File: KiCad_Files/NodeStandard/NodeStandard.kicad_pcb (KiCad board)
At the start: 2 copper layers, 105 parts, among them J1 AC Current In, J10 Opto Coupler 1 in, J11 Opto Coupler 2 in, J12 Opto Coupler 3 in, J13 Relay 1 Output, J14 Relay 2 Output, J15 Schakelaar 3 in, J16 Schakelaar 2 in, J17 Schakelaar 1 in, J18 Force output FET 1 on, J19 Force output FET 2 on, J2 AudioJack3_SwitchTR, J20 FET 1 Output, J21 FET 1 Output, J22 Force output Relay 3 on, J23 Relay 3 Output 1, J24 Relay 3 Output 2, J25 230VAC in, J26 5V-in, J27 ExtDC-in, J3 AC Current loop, J4 EXT1, J5 OledDisplay, J6 RFIDReader, J7 EXT2, J8 Force output Relay 1 on, J9 Force output Relay 2 on, K1 SANYOU_SRD_Form_C, K2 SANYOU_SRD_Form_C, K3 RT42xAxx, Q1 BC547, Q2 BC547, Q3 IRLZ34N, Q4 IRLZ34N, Q5 BC547, U1 MCP23017_SP

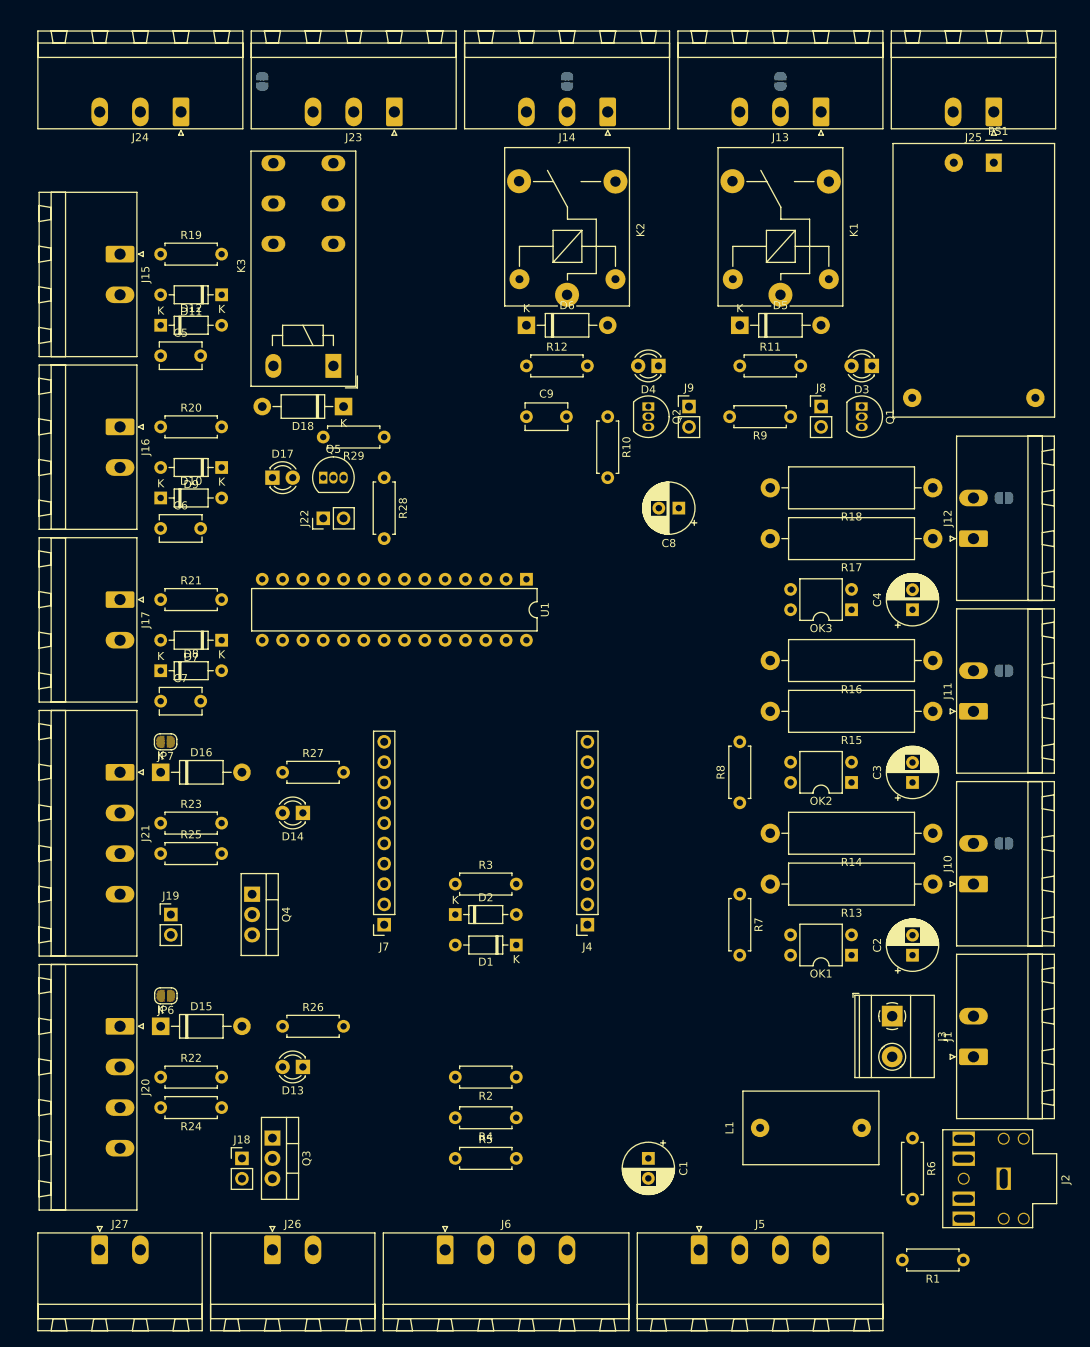
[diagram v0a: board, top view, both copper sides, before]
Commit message: V0.5 Work in progress, first version  PCB design, no silk screen yet
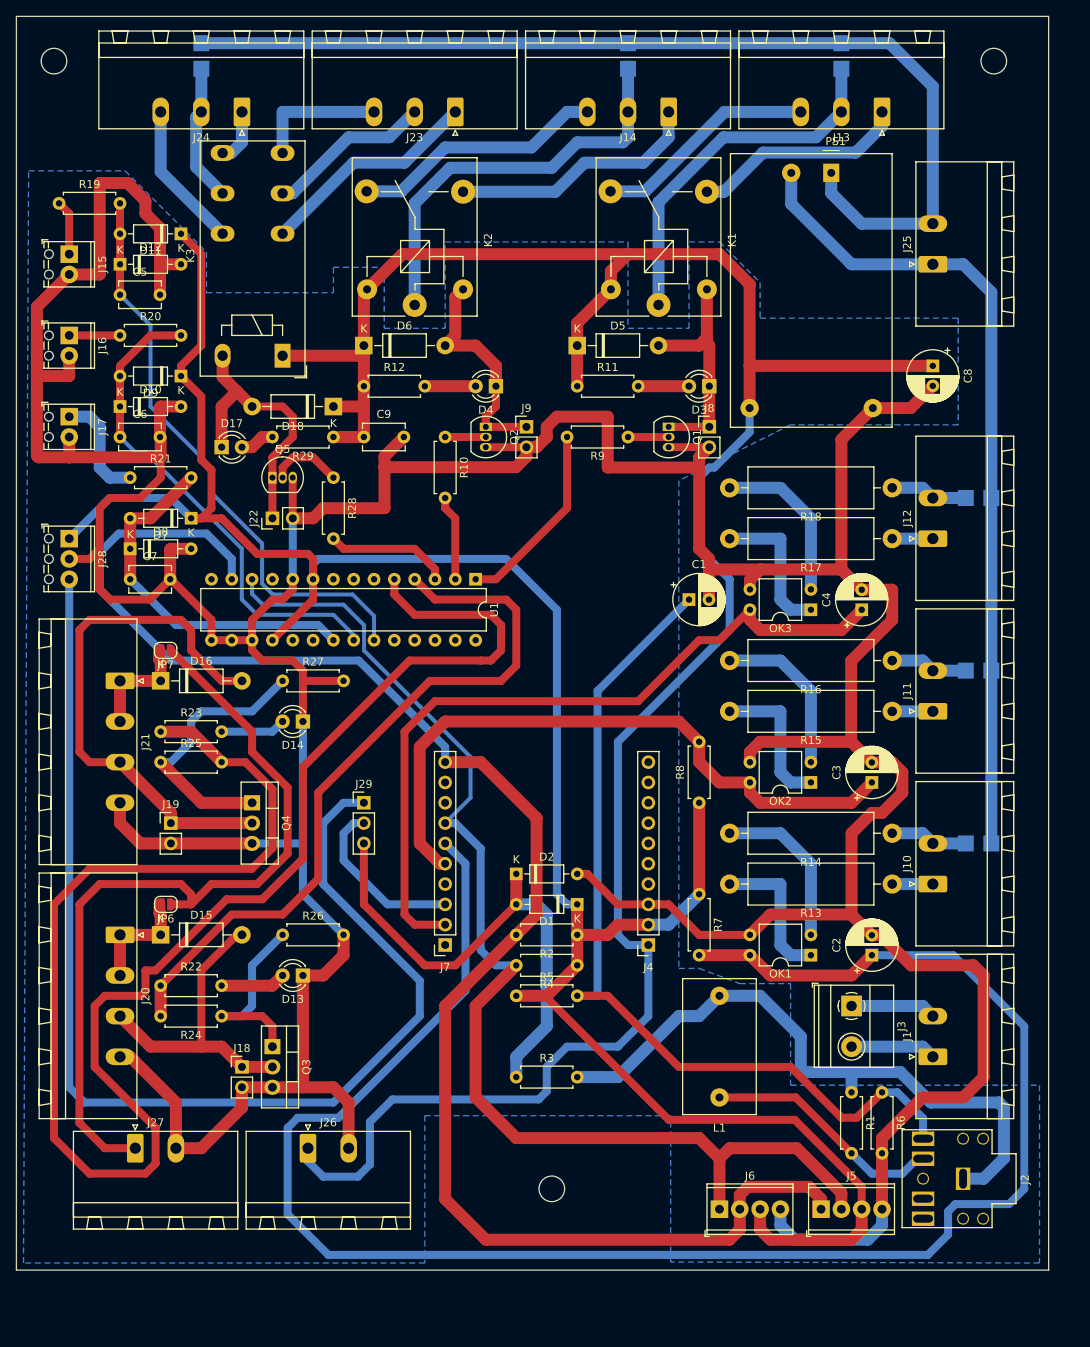
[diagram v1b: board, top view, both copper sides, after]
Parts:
- added J28: Hal current sensor, TerminalBlock_Phoenix:TerminalBlock_Phoenix_MPT-0,5-3-2.54_1x03_P2.54mm_Horizontal, F.Cu at (36.8, 86.4)
- added J29: Current sensor select, Connector_PinHeader_2.54mm:PinHeader_1x03_P2.54mm_Vertical, F.Cu at (73.7, 119.4)
- added REF**: MountingHole_3.2mm_M3, MountingHole:MountingHole_3.2mm_M3, F.Cu at (97.2, 167.6)
- added REF**: MountingHole_3.2mm_M3, MountingHole:MountingHole_3.2mm_M3, F.Cu at (152.4, 26.7)
- added REF**: MountingHole_3.2mm_M3, MountingHole:MountingHole_3.2mm_M3, F.Cu at (34.9, 26.7)
- J15, J16, J17: footprint Connector_Phoenix_MSTB:PhoenixContact_MSTB_2,5_2-GF-5,08_1x02_P5.08mm_Horizontal_ThreadedFlange -> TerminalBlock_Phoenix:TerminalBlock_Phoenix_MPT-0,5-2-2.54_1x02_P2.54mm_Horizontal
- J5, J6: footprint Connector_Phoenix_MSTB:PhoenixContact_MSTB_2,5_4-GF-5,08_1x04_P5.08mm_Horizontal_ThreadedFlange -> TerminalBlock_Phoenix:TerminalBlock_Phoenix_MPT-0,5-4-2.54_1x04_P2.54mm_Horizontal
- JP1, JP2, JP3, JP4, JP5, JP8: footprint Jumper:SolderJumper-2_P1.3mm_Open_RoundedPad1.0x1.5mm -> Footprints:SolderJumper-2_P3mm_Open_RoundedPad
- moved C1 70.0 mm to (114.3, 94.0), turned to 0 degrees
- moved C8 36.4 mm to (144.8, 64.8), turned to 270 degrees
- moved J6 34.7 mm to (118.1, 170.2)
- moved R3 25.3 mm to (92.7, 153.7)
- moved R1 25.2 mm to (134.6, 155.6), turned to 270 degrees
- moved Q1 24.3 mm to (111.8, 72.4)
- moved J17 23.7 mm to (36.8, 71.1)
- moved R5 21.7 mm to (92.7, 143.5)
- moved R4 20.5 mm to (100.3, 139.7)
- moved J25 20.5 mm to (144.8, 52.1), turned to 90 degrees
- moved C9 20.5 mm to (73.7, 73.7)
- moved D5 20.5 mm to (100.3, 62.2)
- moved D6 20.5 mm to (73.7, 62.2)
- moved R10 20.5 mm to (83.8, 73.7)
- moved R11 20.5 mm to (100.3, 67.3)
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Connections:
- D1 pad 2: GPI35 -> Net-(D1-Pad2)
- D2 pad 1: GPI35 -> Net-(D1-Pad2)
- J25 pad 1: 230VAC-L -> 230VAC-N
- J25 pad 2: 230VAC-N -> 230VAC-L
- R3 pad 1: GPI35 -> Net-(D1-Pad2)
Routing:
- net GND: track 0.00 -> 661.1 mm
- net +5V: track 0.00 -> 292.8 mm
- net +3V3: track 0.00 -> 279.6 mm
- net GPIO32: track 0.00 -> 225.6 mm
- net FET2: track 0.00 -> 219.7 mm
- net GPIO13_I2C-SDA: track 0.00 -> 202.1 mm
- net GPIO16_I2C-SCL: track 0.00 -> 151.4 mm
- net Net-(J28-Pad3): track 0.00 -> 147.8 mm
- net 230VAC-L: track 0.00 -> 127.6 mm
- net Net-(C1-Pad1): track 0.00 -> 111.6 mm
- net 230VAC-N: track 0.00 -> 102.4 mm
- net ExternalDCPower: track 0.00 -> 101.1 mm
- net GPI36_U1RXD: track 0.00 -> 94.8 mm
- net FET1: track 0.00 -> 92.4 mm
- net GPIO33: track 0.00 -> 81.6 mm
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- added copper zone on B.Cu, net GND
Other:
- board outline added: 129 x 156.7 mm
